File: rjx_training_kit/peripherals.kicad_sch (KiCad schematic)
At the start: 51 parts, among them J4 LiPo_4.2V, J5 LiPo_4.2V, Q1 BC817, Q2 BC808, Q3 BC817, Q4 BC817, SW2 SW_Push, U3 TMP1075DGK, U4 MCP2562-E-SN, U5 BQ24072RGT, U6 BQ27441-G1, U7 KCSA02-136, U8 LIS3DH

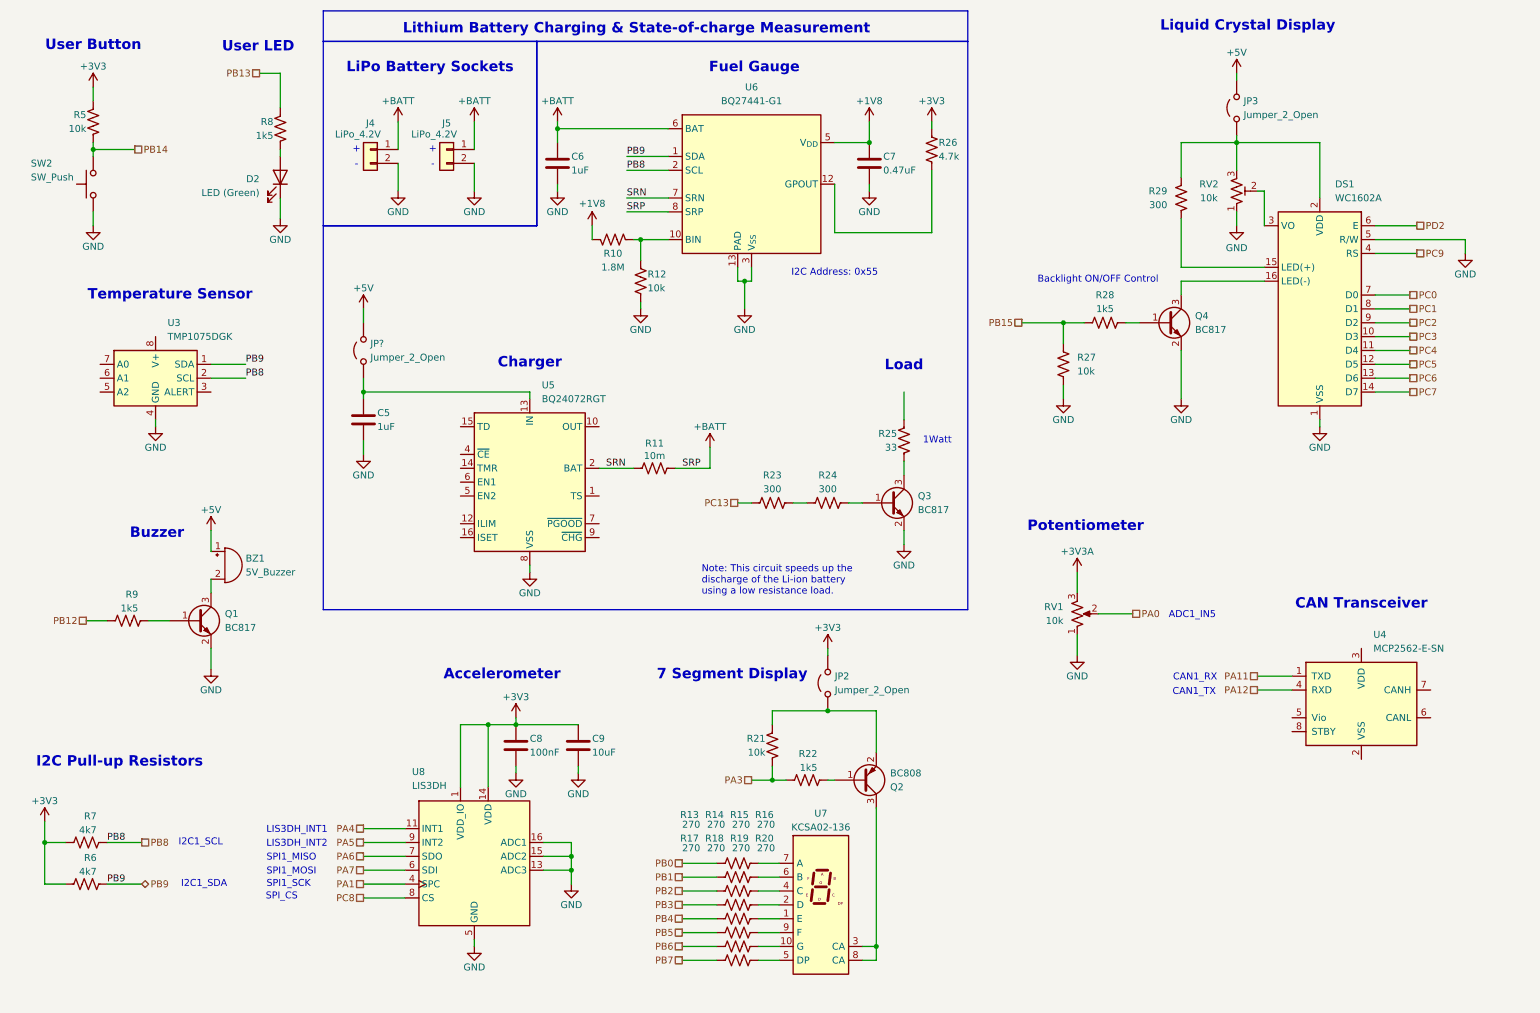
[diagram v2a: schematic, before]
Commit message: Update
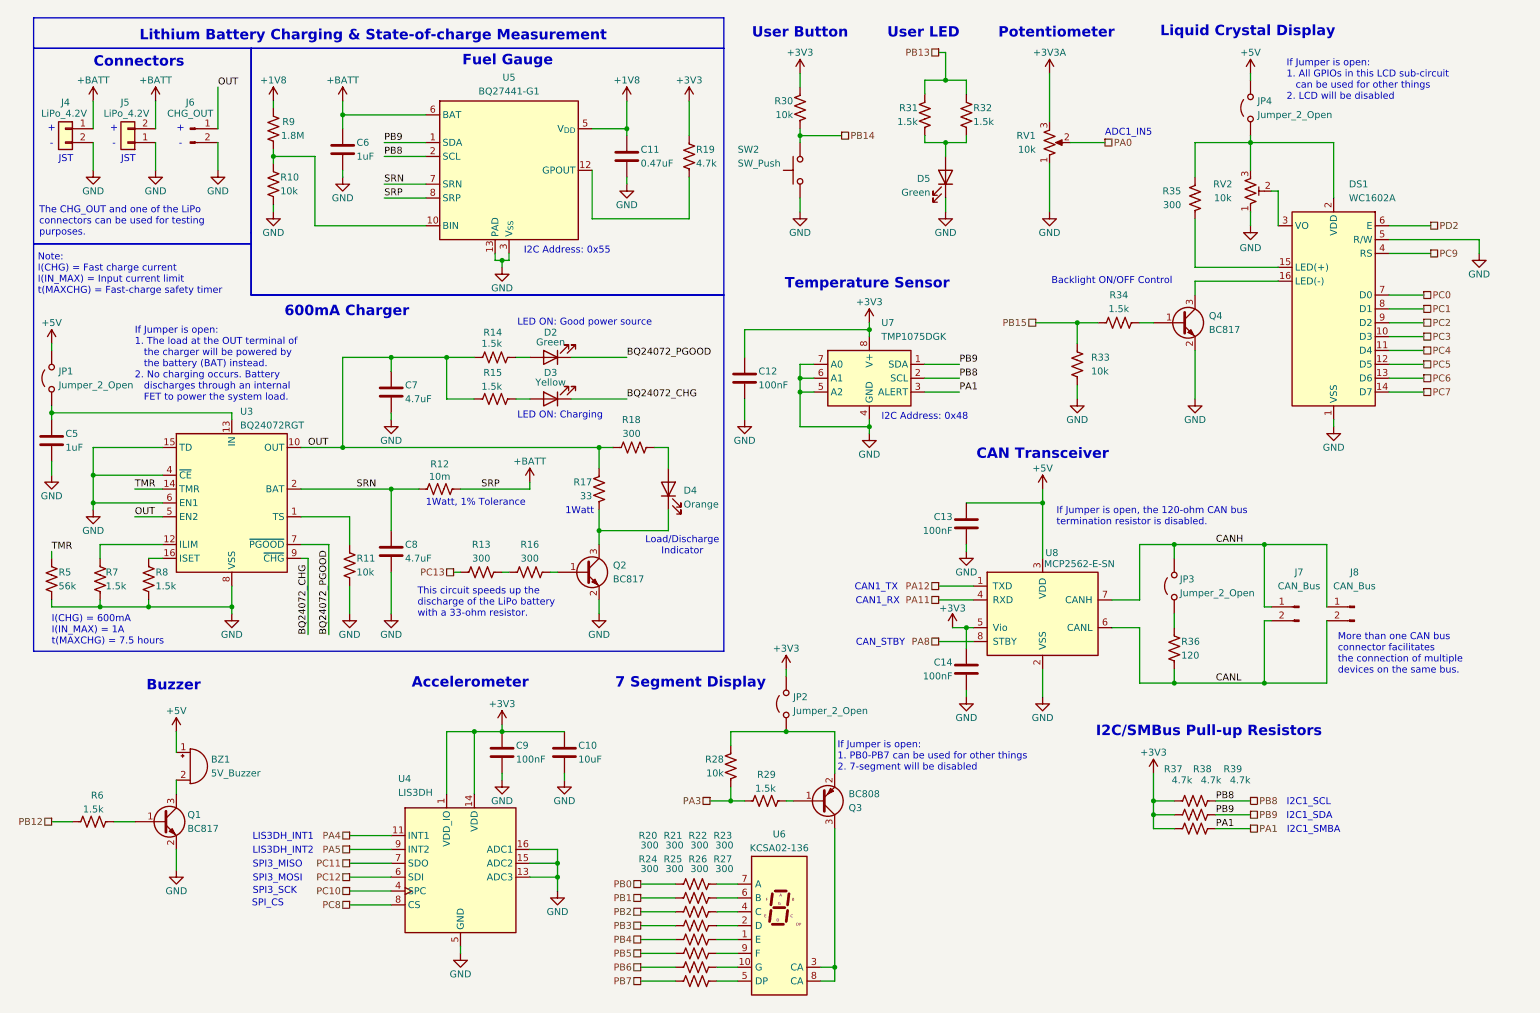
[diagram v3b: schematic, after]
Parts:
- added C12, C13, C14: 100nF, symbol Device:C
- added C7, C8: 4.7uF, symbol Device:C
- added D2: Green, symbol Device:LED
- added D3: Yellow, symbol Device:LED
- added D4: Orange, symbol Device:LED
- added J6: CHG_OUT, symbol Connector:Conn_01x02_Pin
- added J7, J8: CAN_Bus, symbol Connector:Conn_01x02_Pin
- added JP3: Jumper_2_Open, symbol Jumper:Jumper_2_Open
- added R11: 10k, symbol Device:R_US
- added R14, R15, R32, R7, R8: 1.5k, symbol Device:R_US
- added R18: 300, symbol Device:R_US
- added R36: 120, symbol Device:R_US
- added R39: 4.7k, symbol Device:R_US
- added R5: 56k, symbol Device:R_US
- D5: renamed from D2; value LED (Green) -> Green
- R20: renamed from R13; value 270 -> 300
- R21: renamed from R14; value 270 -> 300
- R22: renamed from R15; value 270 -> 300
- R23: renamed from R16; value 270 -> 300
- R24: renamed from R17; value 270 -> 300
- R25: renamed from R18; value 270 -> 300
- R26: renamed from R19; value 270 -> 300
- R27: renamed from R20; value 270 -> 300
- R29: renamed from R22; value 1k5 -> 1.5k
- R31: renamed from R8; value 1k5 -> 1.5k
- R34: renamed from R28; value 1k5 -> 1.5k
- R37: renamed from R7; value 4k7 -> 4.7k
- R38: renamed from R6; value 4k7 -> 4.7k
- R6: renamed from R9; value 1k5 -> 1.5k
- gave numbers to parts that had none: 1
- renumbered C9 to C10, C7 to C11, C8 to C9, JP3 to JP4, Q3 to Q2, Q2 to Q3, R12 to R10, R11 to R12, R23 to R13, R24 to R16, R25 to R17, R26 to R19, R21 to R28, R5 to R30, R27 to R33, R29 to R35, R10 to R9, U5 to U3, U8 to U4, U6 to U5, U7 to U6, U3 to U7, U4 to U8
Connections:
- net +3V3: now also U7.8 (V+), U8.5 (Vio), C12.1, C14.1, R39.1
- net +5V: now also U8.3 (VDD), C13.1
- net +BATT: now also J5.2 (Pin_2); no longer J5.1 (Pin_1)
- net GND: now also J5.1 (Pin_1), U3.15 (TD), U3.4 (~{CE}), U3.6 (EN1), U7.5 (A2), U7.6 (A1), U7.7 (A0), U8.2 (VSS), C12.2, C13.2, C14.2, C7.2, C8.2, J6.2 (Pin_2), R11.2, R5.2, R7.2, R8.2; no longer J5.2 (Pin_2)
- net PA1: now also U7.3 (ALERT), R39.2; no longer U4.4 (SPC)
- net PA11: now also U8.4 (RXD); no longer U8.1 (TXD)
- net PA12: now also U8.1 (TXD); no longer U8.4 (RXD)
- net PB13: now also R32.1
- net SRN: now also C8.1
- net at D5.2 (A), R31.2: now also R32.2
- net at Q2.3 (C), R17.2: now also D4.1 (K)
- net OUT: now reaches R17.1
- net OUT: now also U3.10 (OUT), U3.11 (OUT), U3.5 (EN2), C7.1, J6.1 (Pin_1), R14.1, R15.1, R18.1
- net CANL: now reaches U8.6 (CANL)
- net CANL: now also J7.2 (Pin_2), J8.2 (Pin_2), R36.2
- net CANH: now reaches U8.7 (CANH)
- net CANH: now also J7.1 (Pin_1), J8.1 (Pin_1), JP3.2 (B)
- net PA8: now reaches U8.8 (STBY)
- net at U3.1 (TS): now also R11.1
- net at U3.12 (ILIM): now also R7.1
- net TMR: now reaches U3.14 (TMR)
- net TMR: now also R5.1
- net at U3.16 (ISET): now also R8.1
- net BQ24072_PGOOD: now reaches U3.7 (~{PGOOD})
- net BQ24072_PGOOD: now also D2.1 (K)
- net BQ24072_CHG: now reaches U3.9 (~{CHG})
- net BQ24072_CHG: now also D3.1 (K)
- net PA6 renamed PC11
- net PA7 renamed PC12
- new net: D2.2 (A), R14.2
- new net: JP3.1 (A), R36.1
- new net: D4.2 (A), R18.2
- new net: D3.2 (A), R15.2
- new net PC10: U4.4 (SPC)
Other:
- note added: "1Watt, 1% Tolerance"
- note added: "600mA Charger"
- note added: "CAN_STBY"
- note added: "Connectors"
- note added: "I(CHG) = 600mA I(IN_MAX) = 1A t(MAXCHG) = 7.5 hours"
- note added: "I2C Address: 0x48"
- note added: "I2C/SMBus Pull-up Resistors"
- note added: "I2C1_SMBA"
- note added: "If Jumper is open, the 120-ohm CAN bus termination resistor is disabled."
- note added: "If Jumper is open: 1. All GPIOs in this LCD sub-circuit can be used for other things 2. LCD will be disabled"
- note added: "If Jumper is open: 1. PB0-PB7 can be used for other things 2. 7-segment will be disabled"
- note added: "If Jumper is open: 1. The load at the OUT terminal of the charger will be powered by the battery (BAT) instead. 2. No charging occurs. Battery discharges through an internal FET to power the system load."
- note added: "JST"
- note added: "LED ON: Charging"
- note added: "LED ON: Good power source"
- note added: "Load/Discharge Indicator"
- note added: "More than one CAN bus connector facilitates the connection of multiple devices on the same bus."
- note added: "Note: I(CHG) = Fast charge current I(IN_MAX) = Input current limit t(MAXCHG) = Fast-charge safety timer"
- note added: "SPI3_MISO"
- note added: "SPI3_MOSI"
- note added: "SPI3_SCK"
- note added: "The CHG_OUT and one of the LiPo connectors can be used for testing purposes."
- note added: "This circuit speeds up the discharge of the LiPo battery with a 33-ohm resistor."
- note removed: "Charger"
- note removed: "I2C Pull-up Resistors"
- note removed: "LiPo Battery Sockets"
- note removed: "Load"
- note removed: "Note: This circuit speeds up the discharge of the Li-ion battery using a low resistance load."
- note removed: "SPI1_MISO"
- note removed: "SPI1_MOSI"
- note removed: "SPI1_SCK"
- moved on the sheet: BZ1, C10, C11, C5, C6, C9, D5, DS1, J4, J5, JP1, JP2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
